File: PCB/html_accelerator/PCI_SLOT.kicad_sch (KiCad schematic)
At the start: 3 parts, among them J2 Bus_PCI_Express_x8, J3 PCIexpress_bracket, U1 MCS9990

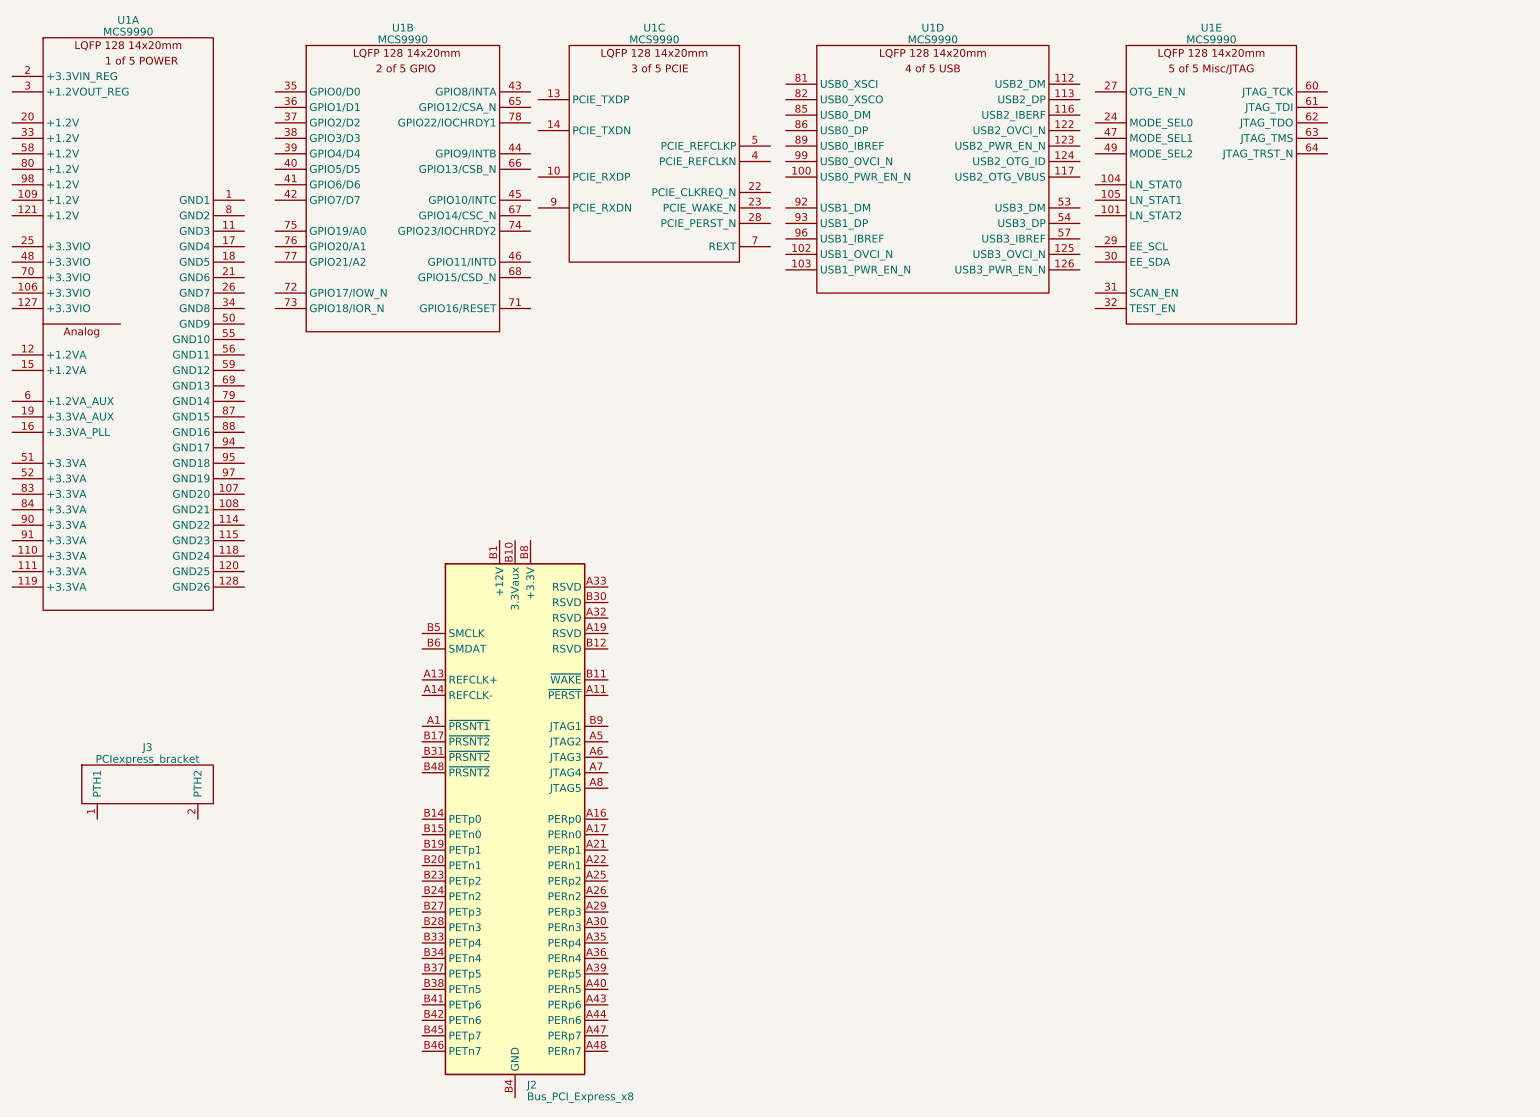
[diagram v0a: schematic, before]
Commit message: Schematic edits
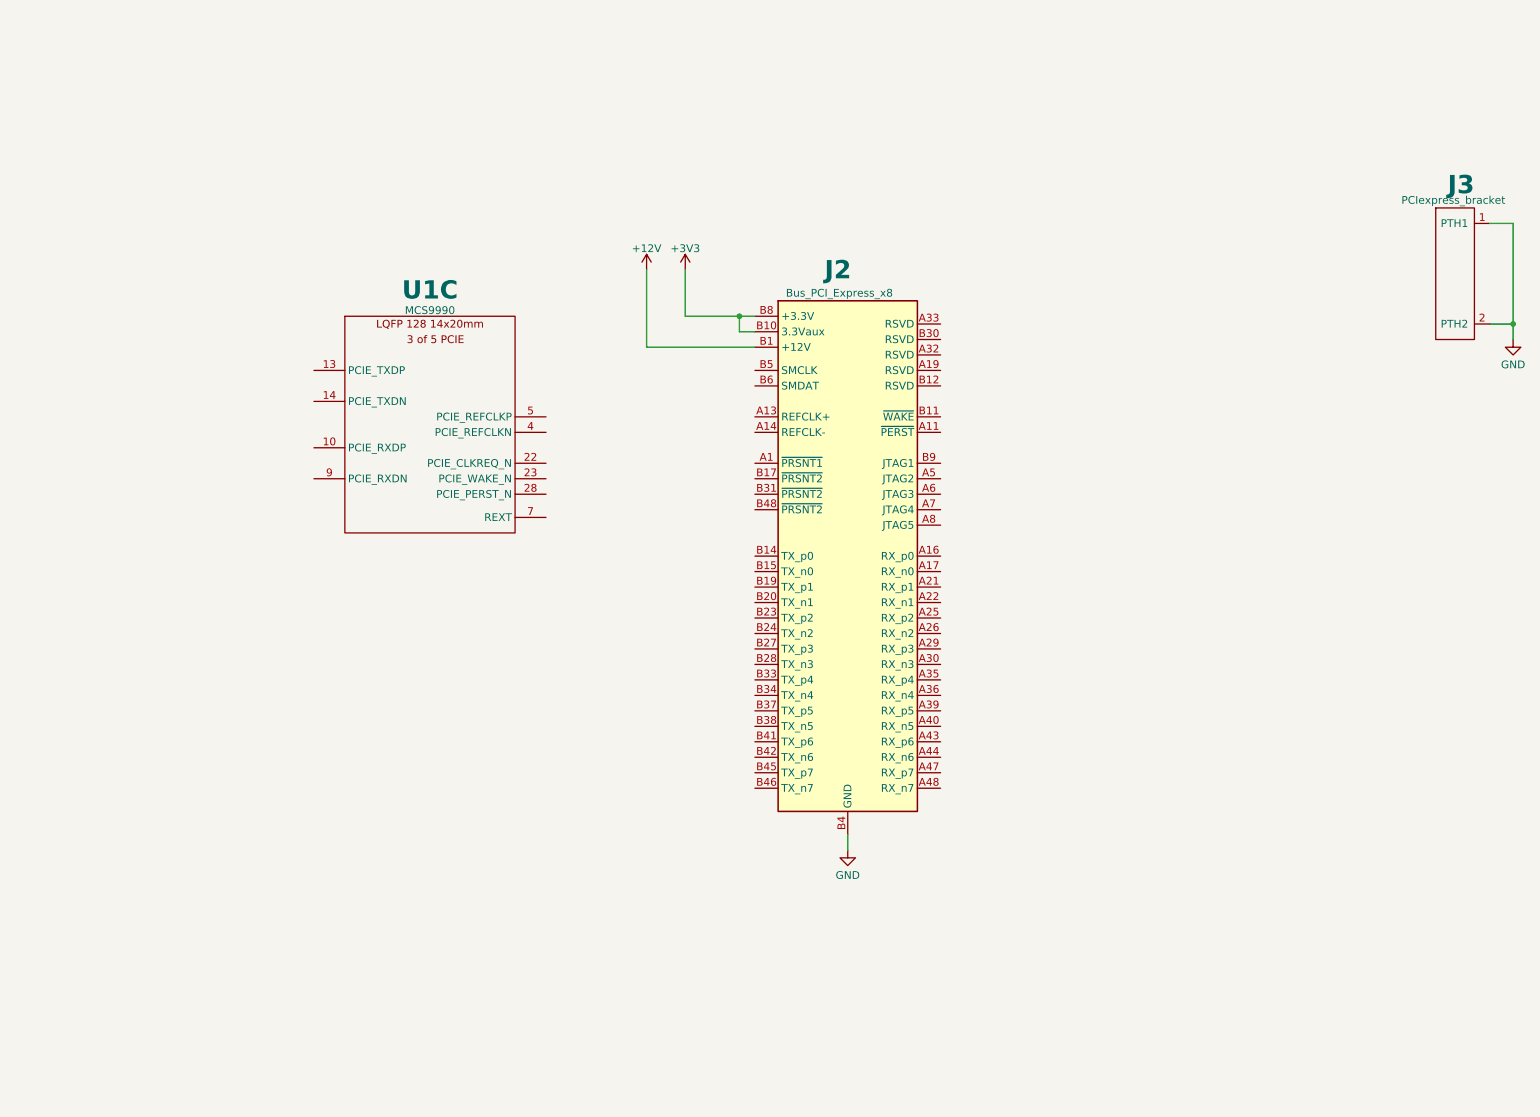
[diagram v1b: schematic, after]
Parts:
- removed unit 5 of U1
- removed unit 4 of U1
- removed unit 2 of U1
- removed unit 1 of U1
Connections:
- net GND: now reaches J3.1 (PTH1)
- net GND: now also J2.A12 (GND), J2.A15 (GND), J2.A18 (GND), J2.A20 (GND), J2.A23 (GND), J2.A24 (GND), J2.A27 (GND), J2.A28 (GND), J2.A31 (GND), J2.A34 (GND), J2.A37 (GND), J2.A38 (GND), J2.A4 (GND), J2.A41 (GND), J2.A42 (GND), J2.A45 (GND), J2.A46 (GND), J2.A49 (GND), J2.B13 (GND), J2.B16 (GND), J2.B18 (GND), J2.B21 (GND), J2.B22 (GND), J2.B25 (GND), J2.B26 (GND), J2.B29 (GND), J2.B32 (GND), J2.B35 (GND), J2.B36 (GND), J2.B39 (GND), J2.B4 (GND), J2.B40 (GND), J2.B43 (GND), J2.B44 (GND), J2.B47 (GND), J2.B49 (GND), J2.B7 (GND), J3.2 (PTH2)
- net +3V3: now reaches J2.A10 (+3.3V), J2.A9 (+3.3V), J2.B8 (+3.3V)
- net +3V3: now also J2.B10 (3.3Vaux)
- net +12V: now reaches J2.A2 (+12V), J2.A3 (+12V), J2.B1 (+12V), J2.B2 (+12V), J2.B3 (+12V)
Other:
- moved on the sheet: J2, J3, U1C
